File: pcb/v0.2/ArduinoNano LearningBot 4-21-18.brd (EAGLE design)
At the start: 106.9 x 58.9 mm, 19 parts

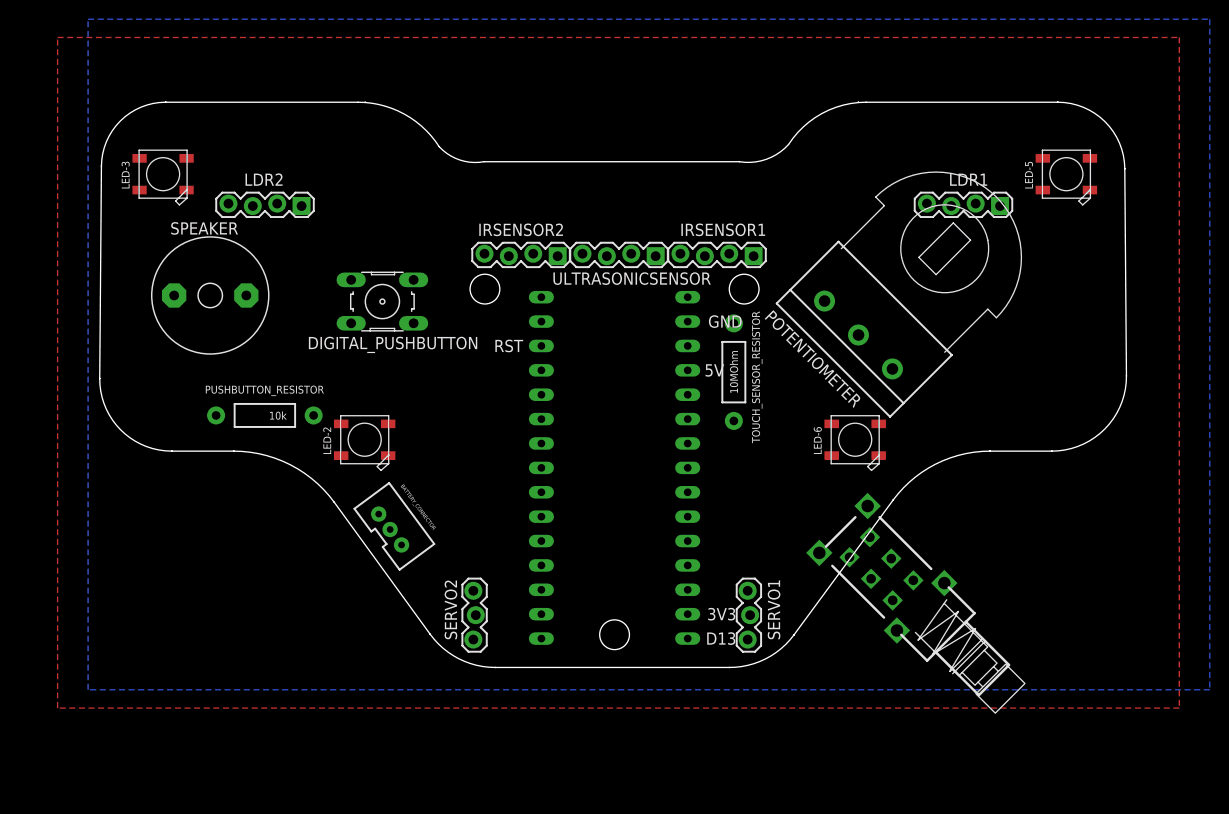
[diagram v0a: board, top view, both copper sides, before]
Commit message: New Board
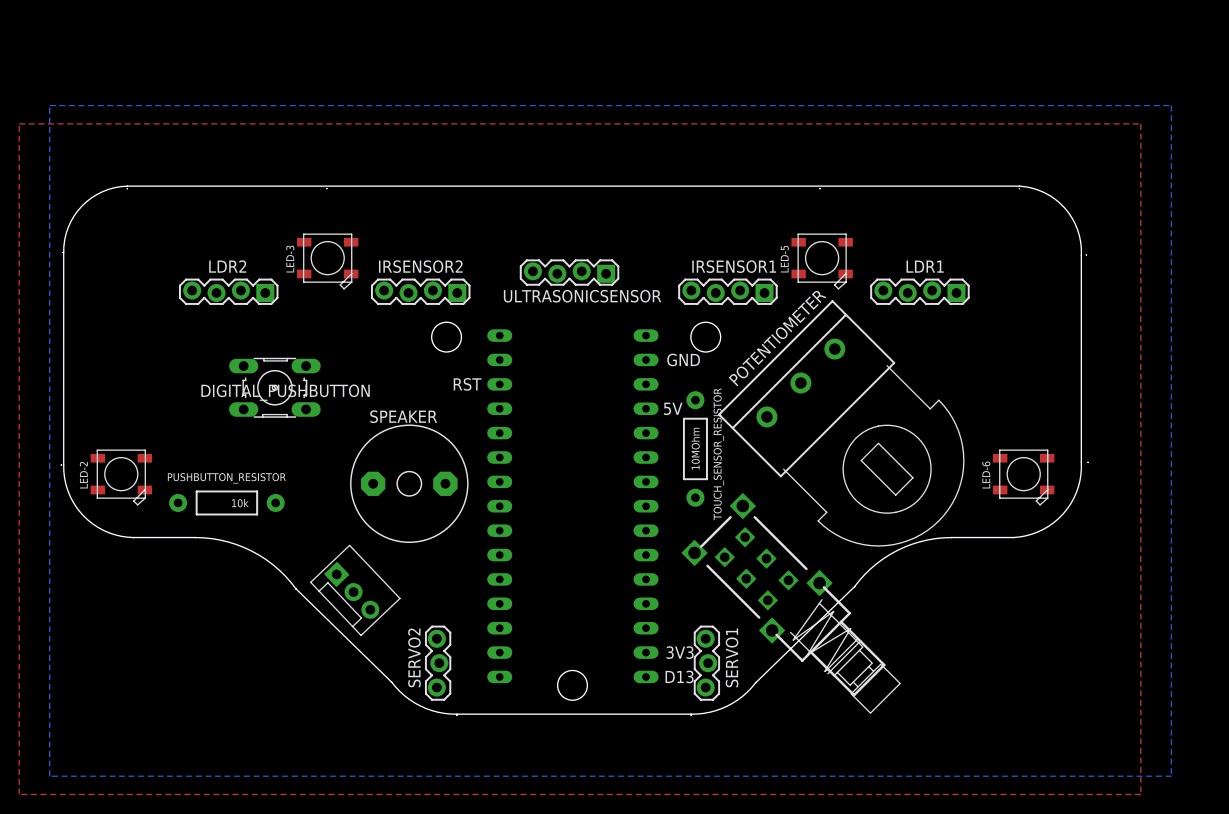
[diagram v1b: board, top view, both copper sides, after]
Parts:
- BATTERY_CONNECTOR: device SparkFun-Connectors:JST-3-PTH-VERT -> SparkFun-Connectors:MOLEX-1X3
- moved SPEAKER 28.5 mm to (36.0, 24.0)
- moved LED-5 26.9 mm to (79.0, 47.5)
- moved LED-2 25.6 mm to (6.00, 25.0)
- moved LED-3 19.2 mm to (27.5, 47.5)
- moved LED-6 17.9 mm to (100.0, 25.0)
- moved DIGITAL_PUSHBUTTON 14.4 mm to (22.0, 34.0)
- moved S1 13.0 mm to (72.0, 15.0)
- moved IRSENSOR2 11.1 mm to (41.0, 44.0)
- moved LDR1 10.1 mm to (93.0, 44.0)
- moved PUSHBUTTON_RESISTOR 9.94 mm to (17.0, 22.0)
- moved LDR2 9.81 mm to (21.0, 44.0)
- moved TOUCH_SENSOR_RESISTOR 8.94 mm to (65.8, 27.6)
- moved POTENTIOMETER 7.81 mm to (76.8, 34.5), turned to 225 degrees
- moved BATTERY_CONNECTOR 7.81 mm to (28.4, 14.6), turned to 313.5 degrees
- moved SERVO1 6.64 mm to (67.0, 2.77)
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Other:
- board size 106.9 x 58.9 mm -> 106.9 x 55.1 mm
